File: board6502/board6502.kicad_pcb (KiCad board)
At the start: 2 copper layers, 48 parts, among them J1 IO Pinheader, J2 UART, J3 USB_B, J4 Expansion Port, J5 Power connector, SW1 Reset button, SW2 SW_NMI, U1 DS1813, U2 74LS00, U3 74LS04, U4 W65C22N, U5 74LS30, U6 W65C51N, U7 W65C02, U8 AT28C64B, U9 CY7C199, X1 1-10MHz, Y1 1.8432M

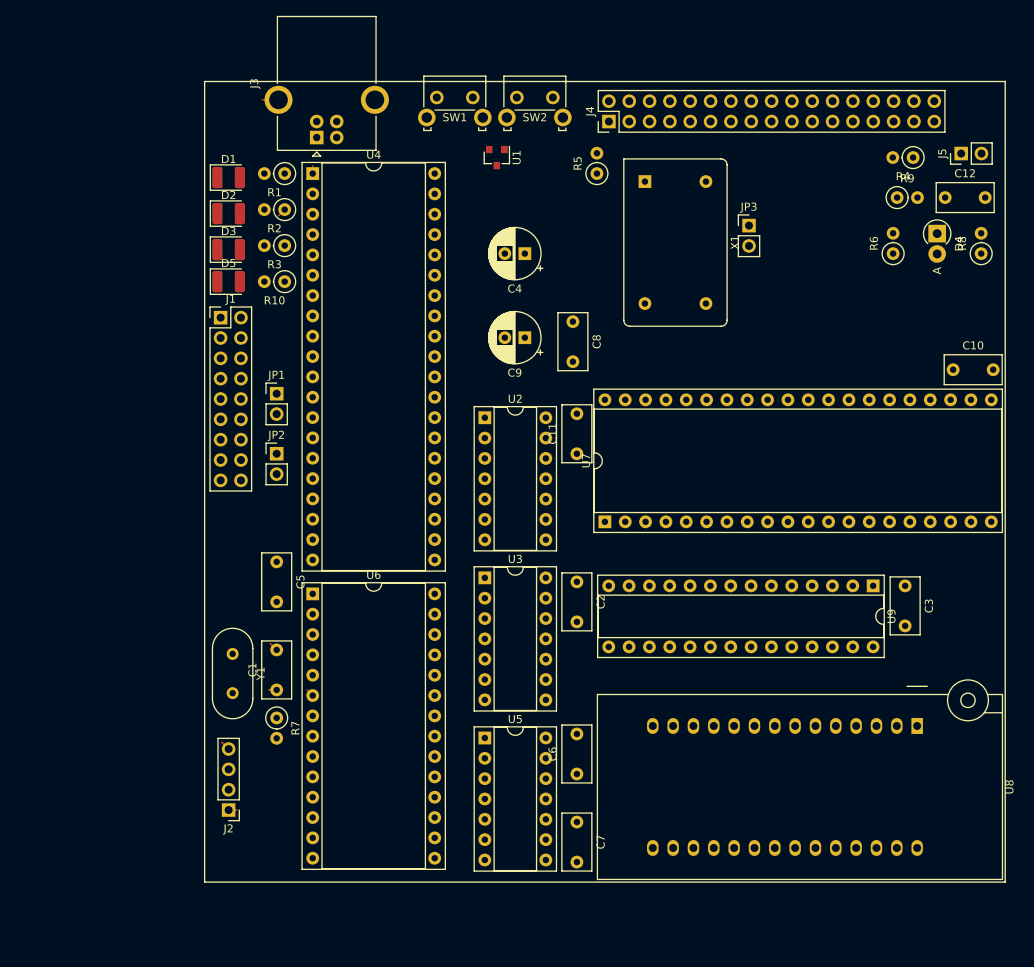
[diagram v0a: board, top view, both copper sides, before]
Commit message: finally complete PCB routing
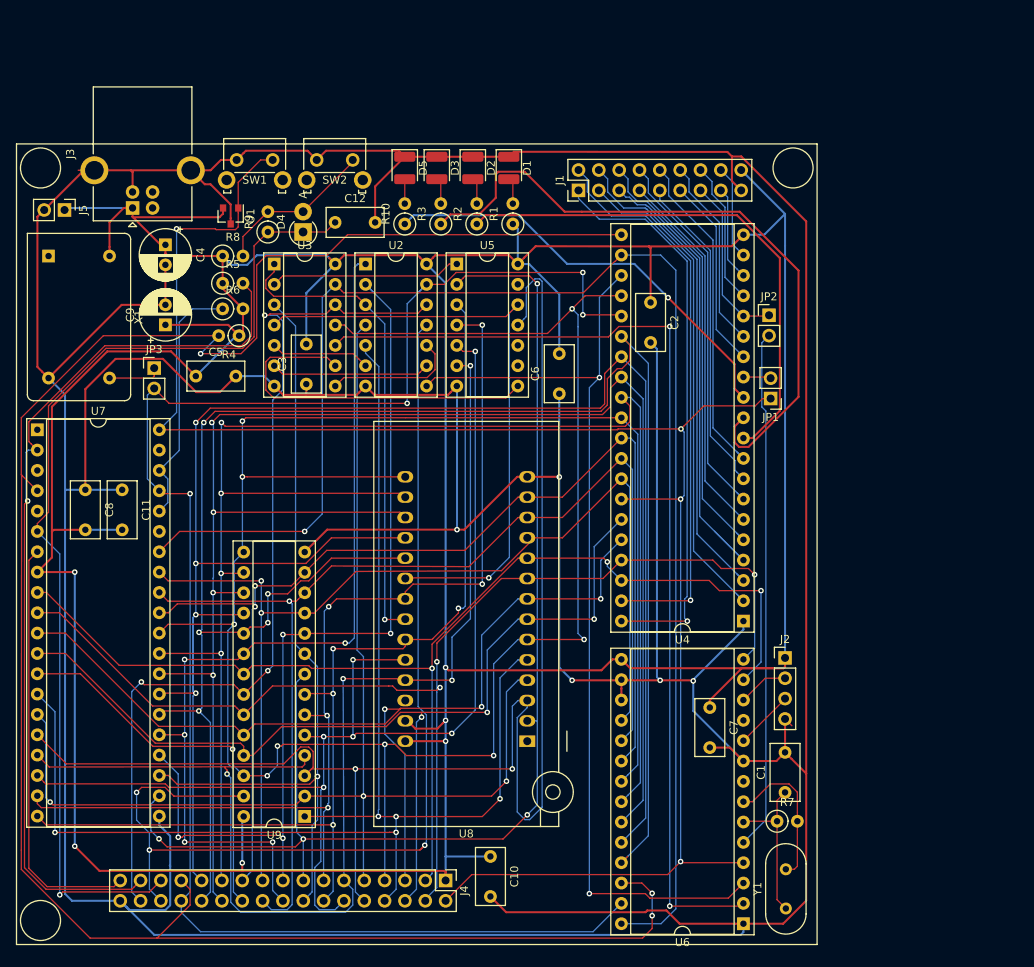
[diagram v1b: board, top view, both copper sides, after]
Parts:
- moved J5 112.2 mm to (102.0, 53.0), turned to 270 degrees
- moved J4 97.0 mm to (149.6, 136.8), turned to 270 degrees
- moved R8 94.8 mm to (121.8, 58.8), turned to 0 degrees
- moved R4 87.1 mm to (123.8, 68.8)
- moved R6 84.0 mm to (121.8, 65.4), turned to 0 degrees
- moved C10 83.9 mm to (155.2, 133.8), turned to 270 degrees
- moved D4 79.2 mm to (131.8, 55.8), turned to 90 degrees
- moved C3 78.9 mm to (132.2, 74.8), turned to 90 degrees
- moved R9 78.7 mm to (127.4, 55.8), turned to 90 degrees
- moved U4 77.6 mm to (186.8, 104.4), turned to 180 degrees
- moved U9 76.6 mm to (132.0, 128.8), turned to 180 degrees
- moved JP3 76.4 mm to (113.2, 72.8)
- moved C12 76.3 mm to (135.8, 54.6)
- moved Y1 76.1 mm to (192.1, 140.3), turned to 90 degrees
- moved X1 75.1 mm to (100.0, 58.8)
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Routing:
- net GND: track 6.24 -> 744.2 mm, vias 0 -> 5
- net +5V: track 2.07 -> 550.3 mm, vias 0 -> 6
- net _IRQ: track 0.00 -> 256.5 mm, vias 0 -> 3
- net D7: track 0.00 -> 229.8 mm, vias 0 -> 5
- net D6: track 0.00 -> 228.2 mm, vias 0 -> 4
- net _RESET: track 0.00 -> 223.9 mm, vias 0 -> 4
- net CLK: track 0.00 -> 208.2 mm, vias 0 -> 4
- net D5: track 0.00 -> 207.8 mm, vias 0 -> 4
- net D4: track 0.00 -> 199.1 mm, vias 0 -> 4
- net A4: track 0.00 -> 188.5 mm, vias 0 -> 7
- net D3: track 0.00 -> 186.3 mm, vias 0 -> 3
- net A7: track 0.00 -> 185.7 mm, vias 0 -> 2
- net RW_: track 0.00 -> 184.7 mm, vias 0 -> 1
- net A5: track 0.00 -> 176.2 mm, vias 0 -> 5
- net A12: track 0.00 -> 159.9 mm, vias 0 -> 4
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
